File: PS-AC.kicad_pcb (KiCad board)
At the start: 2 copper layers, 65 x 50 mm, 20 parts, among them J1 Conn_01x02, J2 Conn_01x02, J3 Conn_01x04, Q1 NTZD3154NT1G, U1 HLK-10M05, U2 INA219AxD, U3 AMS1117-3.3

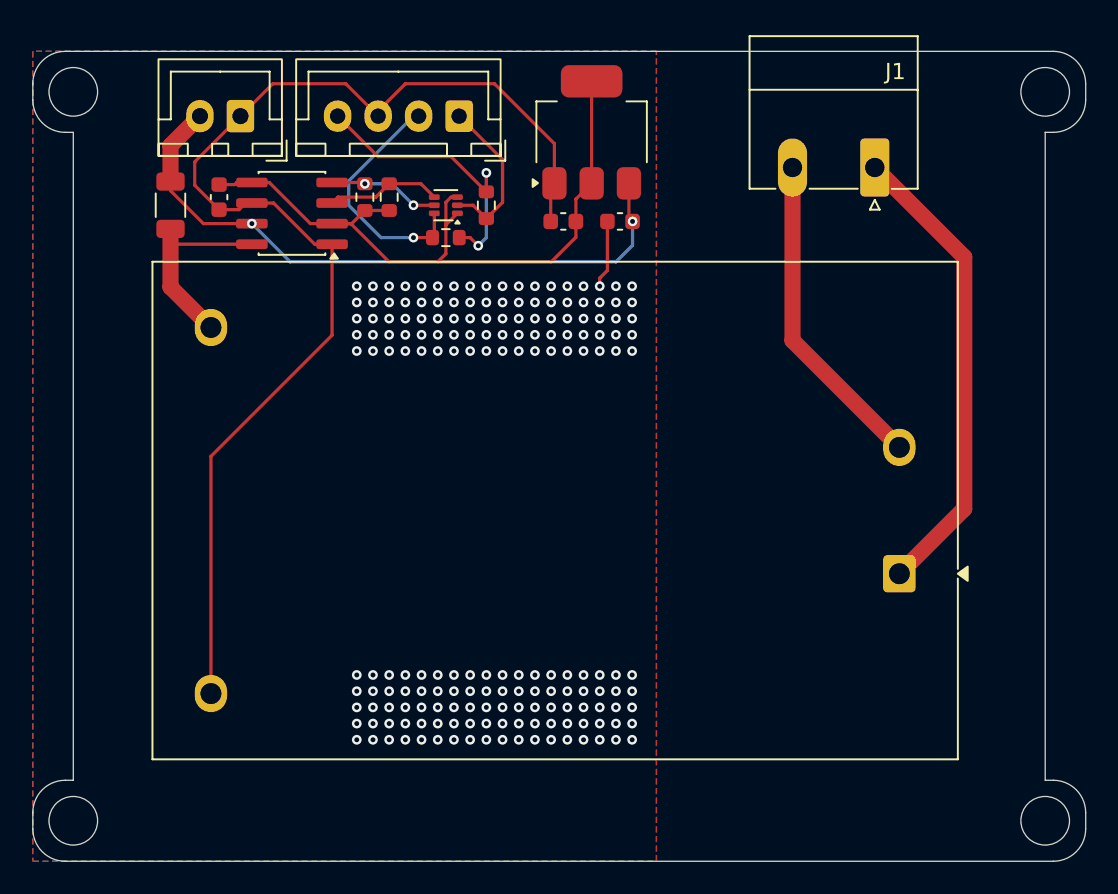
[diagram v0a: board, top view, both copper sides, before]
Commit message: update
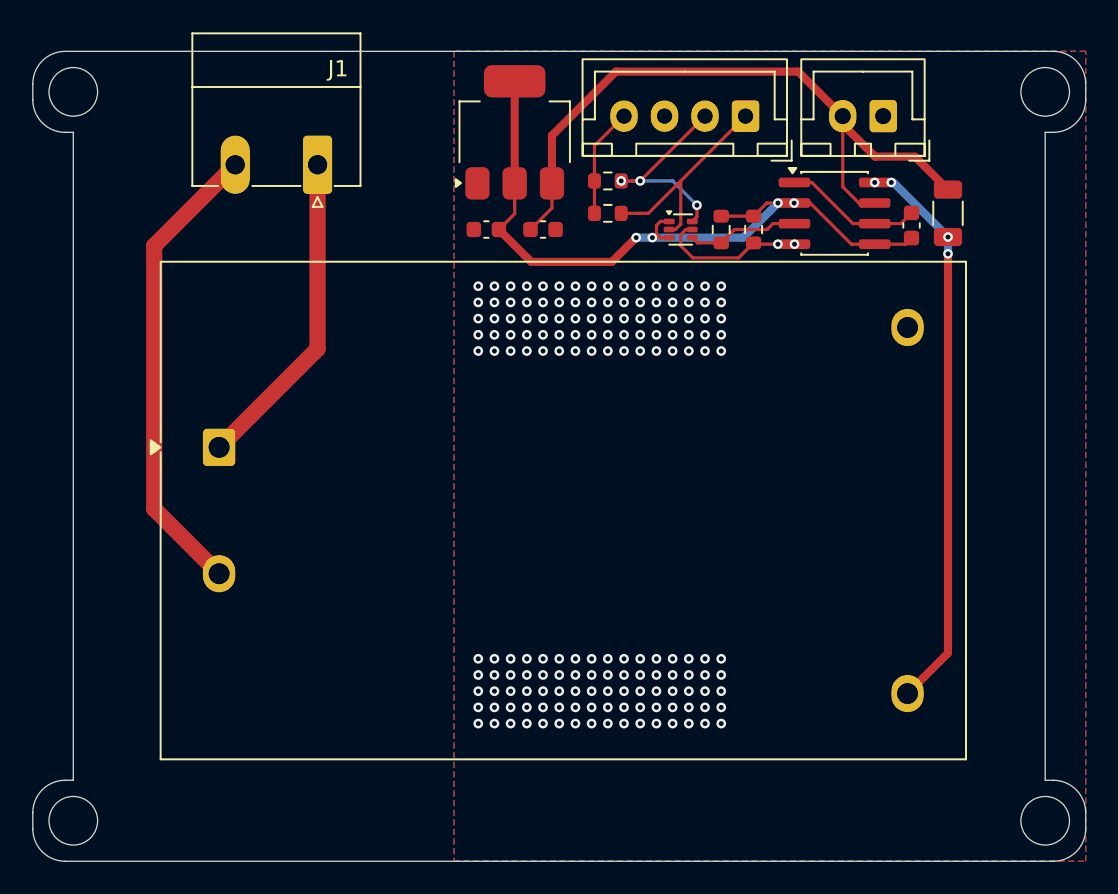
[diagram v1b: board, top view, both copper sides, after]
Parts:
- removed kibuzzard-6A029DFE: G***, kibuzzard-6A029DFE
- moved R1 48.0 mm to (104.0, 57.5)
- moved C1 42.8 mm to (101.8, 58.2), turned to 90 degrees
- moved U1 42.7 mm to (59.0, 71.9), turned to 0 degrees
- moved J2 39.7 mm to (100.0, 51.5)
- moved J1 34.4 mm to (65.1, 54.5)
- moved U2 33.5 mm to (97.0, 57.5), turned to 0 degrees
- moved R3 24.1 mm to (92.0, 58.5), turned to -90 degrees
- moved R5 20.6 mm to (90.0, 58.5), turned to -90 degrees
- moved J3 17.7 mm to (91.5, 51.5)
- moved Q1 14.6 mm to (87.5, 58.5), turned to 0 degrees
- moved R2 10.6 mm to (83.0, 55.5), turned to 0 degrees
- moved R4 7.52 mm to (83.0, 57.5), turned to 0 degrees
- moved C2 4.78 mm to (79.0, 58.5), turned to 180 degrees
- moved C3 4.78 mm to (75.5, 58.5)
- moved U3 4.75 mm to (77.2, 52.5)
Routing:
- net GND: track 79.3 -> 8.55 mm, vias 180 -> 160
- net Net-(U1-+Vout): track 12.8 -> 35.1 mm, vias 0 -> 4
- net VCC: track 18.4 -> 6.76 mm, vias 2 -> 0
- net Net-(J1-Pin_1): track 29.1 -> 20.0 mm
- net Net-(J1-Pin_2): track 20.0 -> 29.0 mm
- net SDA_EXT: track 9.98 -> 13.7 mm
- net SCL: track 6.89 -> 10.3 mm
- net +5V: track 40.0 -> 42.5 mm, vias 2 -> 0
- net +3V3: track 44.4 -> 46.7 mm, vias 0 -> 4
- net SCL_EXT: track 15.0 -> 13.2 mm, vias 1 -> 3
